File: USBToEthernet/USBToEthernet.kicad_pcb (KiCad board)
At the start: 2 copper layers, 61.3 x 30 mm, 54 parts, among them J1 0480372200, J2 L836-1J1T-43, SW1 SW_Push, U1 LAN7500-ABJZ, U2 NCP1117-3.3_SOT223, U3 93LCxxAxxOT, U4 USBLC6-2SC6, U6 AMS1117-1.2, Y1 25Mhz

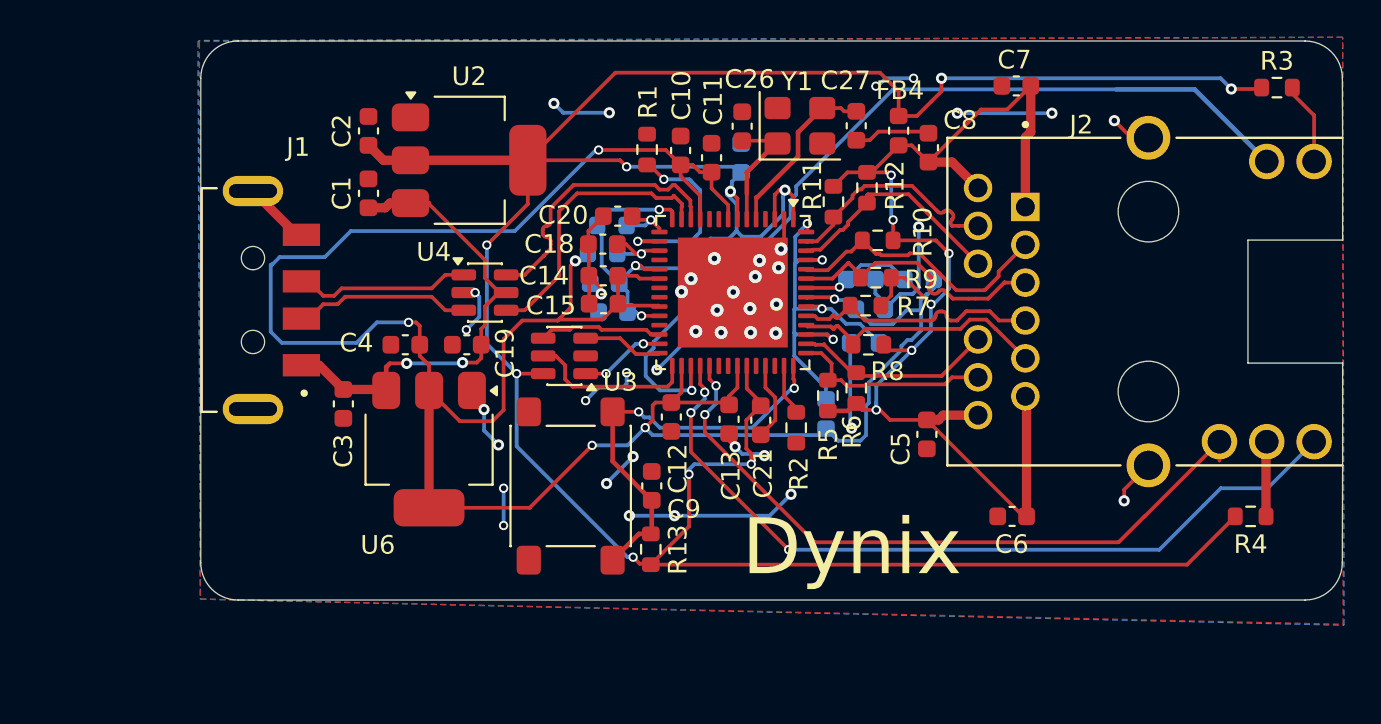
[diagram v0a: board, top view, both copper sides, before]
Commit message: Reroute again
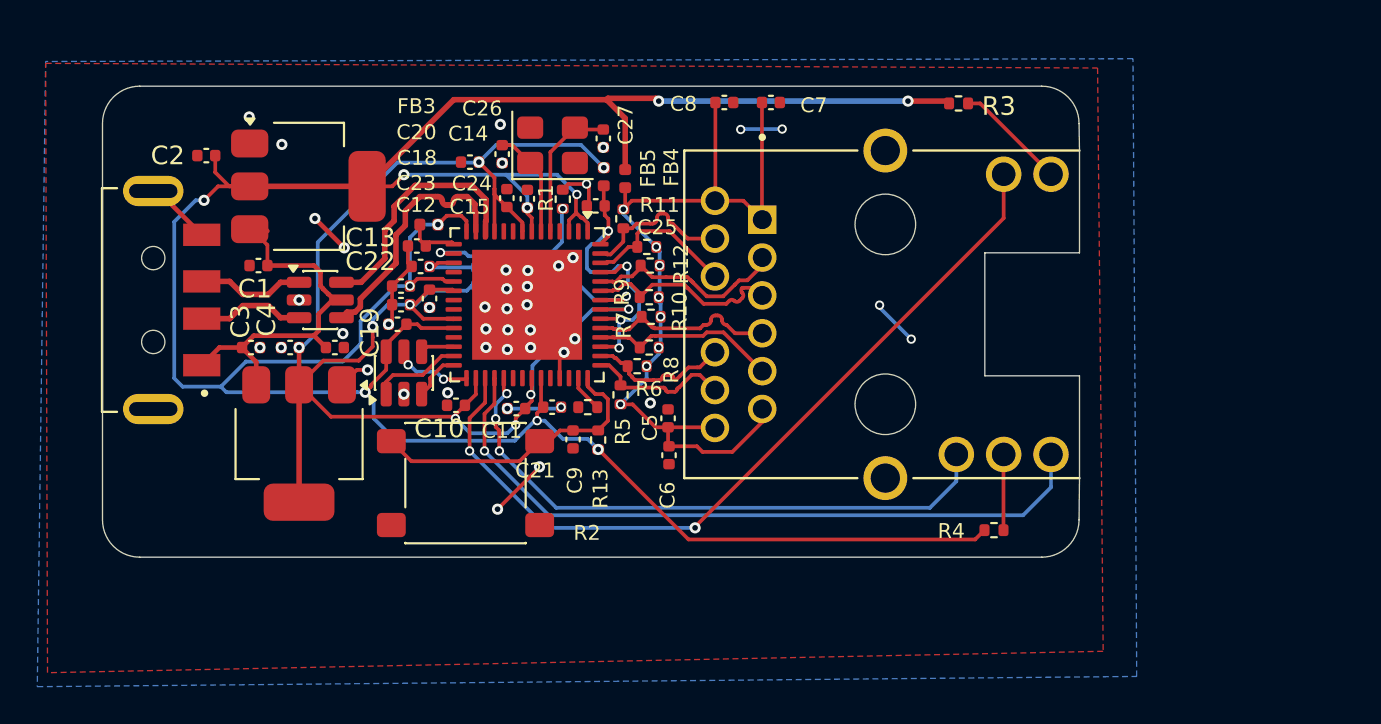
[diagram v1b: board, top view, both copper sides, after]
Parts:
- C1, C10, C11, C12, C13, C14, C15, C16, C17, C18, C19, C2, C20, C21, C26, C27, C3, C4, C5, C6, C7, C8, C9: footprint Capacitor_SMD:C_0603_1608Metric -> Capacitor_SMD:C_0402_1005Metric
- C22, C23, C24, C25: footprint Capacitor_SMD:C_0603_1608Metric -> Capacitor_SMD:C_0402_1005Metric; moved to F.Cu
- FB1, FB2, FB4: footprint Inductor_SMD:L_0603_1608Metric -> Inductor_SMD:L_0402_1005Metric
- FB3, FB5: footprint Inductor_SMD:L_0603_1608Metric -> Inductor_SMD:L_0402_1005Metric; moved to F.Cu
- R1, R10, R11, R12, R13, R2, R3, R4, R5, R6, R7, R8, R9: footprint Resistor_SMD:R_0603_1608Metric -> Resistor_SMD:R_0402_1005Metric
- moved FB1 19.0 mm to (79.3, 88.0)
- moved C6 18.7 mm to (84.9, 96.2), turned to -90 degrees
- moved C10 18.2 mm to (73.4, 93.5), turned to 180 degrees
- moved FB5 17.4 mm to (81.4, 81.3), turned to -90 degrees
- moved C13 17.3 mm to (72.0, 87.8)
- moved R3 17.1 mm to (100.4, 77.3)
- moved C11 17.1 mm to (76.7, 93.7), turned to 180 degrees
- moved C16 16.3 mm to (79.4, 89.1), turned to 180 degrees
- moved C25 16.2 mm to (80.9, 82.8)
- moved C17 15.8 mm to (79.3, 87.0), turned to 180 degrees
- moved C12 15.7 mm to (70.5, 88.2), turned to 180 degrees
- moved FB4 14.9 mm to (82.5, 81.4)
- moved J2 14.1 mm to (96.5, 88.7)
- moved C5 13.9 mm to (84.8, 94.2), turned to 90 degrees
- moved R4 13.8 mm to (102.3, 100.2)
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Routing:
- net GND: track 83.6 -> 30.5 mm, vias 42 -> 43
- net +1V2: track 134.6 -> 86.7 mm, vias 6 -> 9
- net /TR0: track 72.0 -> 46.3 mm, vias 6 -> 8
- net +3V3: track 176.4 -> 160.0 mm, vias 13 -> 11
- net /VBUS: track 27.0 -> 20.4 mm, vias 2 -> 0
- net /RESET: track 22.3 -> 16.6 mm, vias 2 -> 0
- net /VDD12A: track 23.3 -> 17.6 mm
- net /LED2: track 37.3 -> 32.1 mm, vias 2 -> 3
- net /EECLK: track 6.65 -> 1.83 mm
- net /LED1: track 43.2 -> 38.4 mm, vias 3 -> 1
- net /EECS: track 9.01 -> 4.29 mm, vias 0 -> 2
- net /TR2+: track 15.0 -> 10.9 mm
- net /TR3+: track 12.3 -> 8.24 mm
- net /TR3-: track 12.3 -> 8.28 mm
- net /TR2-: track 14.8 -> 10.9 mm
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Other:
- board size 61.3 x 30 mm -> 52.4 x 25.3 mm
